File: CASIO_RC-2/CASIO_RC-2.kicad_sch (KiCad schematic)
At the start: 13 parts, among them J1 Conn_01x21_Pin, J2 Conn_01x02_Pin

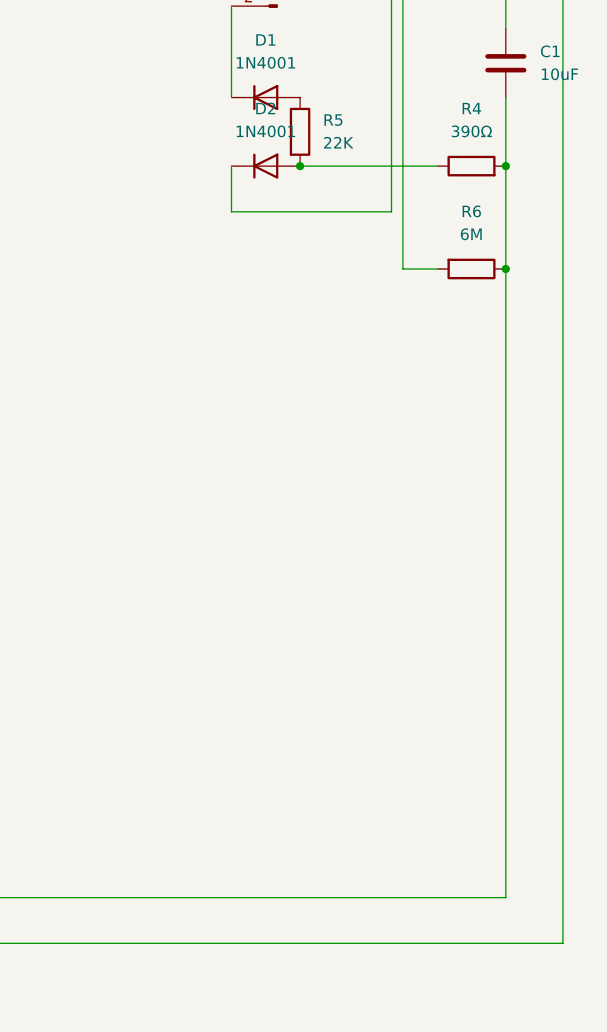
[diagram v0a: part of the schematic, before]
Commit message: Add files via upload
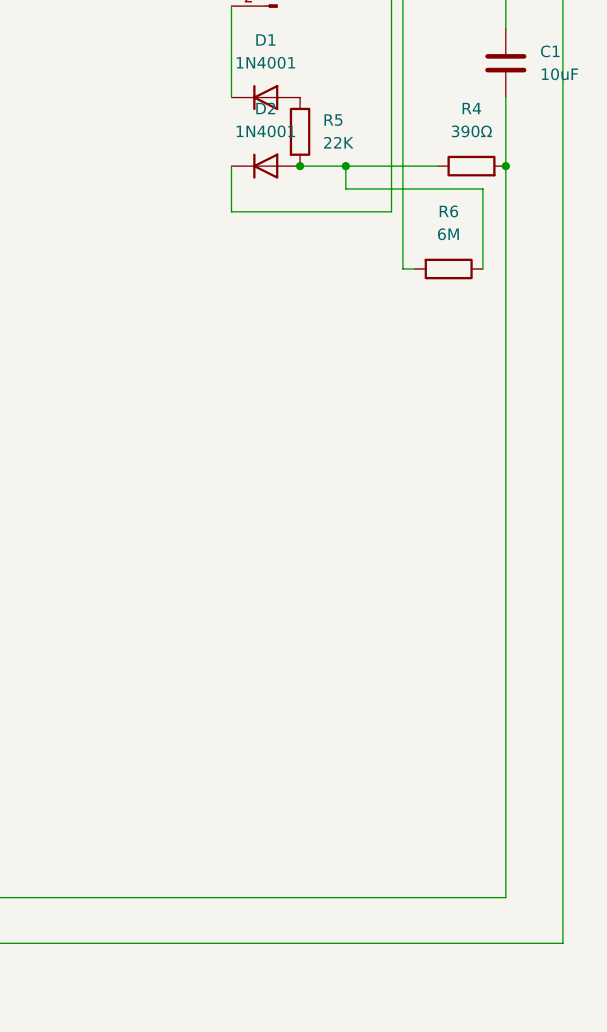
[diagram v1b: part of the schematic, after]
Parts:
- D1, D2: footprint Diode_THT:D_DO-41_SOD81_P10.16mm_Horizontal -> Diode_SMD:D_1206_3216Metric
- J1: footprint (none) -> Custom_Reto_Chips:CASIO_RC-2_RAM_Pinheadder
- J2: footprint (none) -> Custom_Reto_Chips:CR2023_Battery_Terminal
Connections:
- net at C1.2, R4.2, U1.22 (N/C)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: no longer R6.1
- net at D2.2 (A), R4.1, R5.2: now also R6.1
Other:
- moved on the sheet: R6
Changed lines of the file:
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@@
+	)
+	(junction
+		(at 198.12 58.42)
+		(diameter 0)
+		(color 0 0 0 0)
 	)
 	(junction
@@
 	(junction
 		(at 88.9 102.87)
-		(diameter 0)
-		(color 0 0 0 0)
-	)
-	(junction
-		(at 215.9 69.85)
 		(diameter 0)
 		(color 0 0 0 0)
@@
 	(wire
 		(pts
-			(xy 193.04 58.42) (xy 208.28 58.42)
+			(xy 193.04 58.42) (xy 198.12 58.42)
 		)
 		(stroke
@@
 	(wire
 		(pts
+			(xy 198.12 60.96) (xy 198.12 58.42)
+		)
+		(stroke
+			(width 0)
+			(type default)
+		)
+	)
+	(wire
+		(pts
 			(xy 185.42 63.5) (xy 203.2 63.5)
 		)
@@
 	(wire
 		(pts
-			(xy 215.9 58.42) (xy 215.9 69.85)
+			(xy 215.9 58.42) (xy 215.9 139.7)
 		)
 		(stroke
@@
 	(wire
 		(pts
+			(xy 213.36 69.85) (xy 213.36 60.96)
+		)
+		(stroke
+			(width 0)
+			(type default)
+		)
+	)
+	(wire
+		(pts
 			(xy 93.98 119.38) (xy 147.32 119.38)
 		)
@@
 	(wire
 		(pts
+			(xy 198.12 58.42) (xy 208.28 58.42)
+		)
+		(stroke
+			(width 0)
+			(type default)
+		)
+	)
+	(wire
+		(pts
 			(xy 76.2 60.96) (xy 76.2 57.15)
 		)
@@
 	(wire
 		(pts
+			(xy 213.36 60.96) (xy 198.12 60.96)
+		)
+		(stroke
+			(width 0)
+			(type default)
+		)
+	)
+	(wire
+		(pts
 			(xy 215.9 139.7) (xy 93.98 139.7)
 		)
@@
 	(wire
 		(pts
-			(xy 208.28 69.85) (xy 204.47 69.85)
+			(xy 205.74 69.85) (xy 204.47 69.85)
 		)
 		(stroke
@@
 		(pts
 			(xy 83.82 71.12) (xy 60.96 71.12)
-		)
-		(stroke
-			(width 0)
-			(type default)
-		)
-	)
-	(wire
-		(pts
-			(xy 215.9 69.85) (xy 215.9 139.7)
 		)
 		(stroke
@@
 			)
 		)
-		(property "Footprint" ""
+		(property "Footprint" "Custom_Reto_Chips:CR2023_Battery_Terminal"
 			(at 190.5 38.1 0)
 			(effects
@@
 			)
 		)
-		(property "Footprint" "Diode_THT:D_DO-41_SOD81_P10.16mm_Horizontal"
+		(property "Footprint" "Diode_SMD:D_1206_3216Metric"
 			(at 189.23 50.8 0)
 			(effects
@@
 			)
 		)
-		(property "Footprint" ""
+		(property "Footprint" "Custom_Reto_Chips:CASIO_RC-2_RAM_Pinheadder"
 			(at 127 25.4 0)
 			(effects
@@
 			)
 		)
-		(property "Footprint" "Diode_THT:D_DO-41_SOD81_P10.16mm_Horizontal"
+		(property "Footprint" "Diode_SMD:D_1206_3216Metric"
 			(at 189.23 58.42 0)
 			(effects
@@
 	(symbol
 		(lib_id "Device:R")
-		(at 212.09 69.85 270)
+		(at 209.55 69.85 270)
 		(unit 1)
 		(exclude_from_sim no)
@@
 		(fields_autoplaced yes)
 		(property "Reference" "R6"
-			(at 212.09 63.5 90)
+			(at 209.55 63.5 90)
 			(effects
 				(font
@@
 		)
 		(property "Value" "6M"
-			(at 212.09 66.04 90)
+			(at 209.55 66.04 90)
 			(effects
 				(font
@@
 		)
 		(property "Footprint" "Resistor_SMD:R_1206_3216Metric"
-			(at 212.09 68.072 90)
+			(at 209.55 68.072 90)
 			(effects
 				(font
@@
 		)
 		(property "Datasheet" "~"
-			(at 212.09 69.85 0)
+			(at 209.55 69.85 0)
 			(effects
 				(font
@@
 		)
 		(property "Description" "Resistor"
-			(at 212.09 69.85 0)
-			(effects
-				(font
+			(at 209.55 69.85 0)
+			(effects
+				(font
